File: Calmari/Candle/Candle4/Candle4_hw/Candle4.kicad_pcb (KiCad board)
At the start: 2 copper layers, 124 x 15 mm, 56 parts, among them Q1 LED_RGB, SW1 BUTTON, SW2 BUTTON, SW3 BUTTON

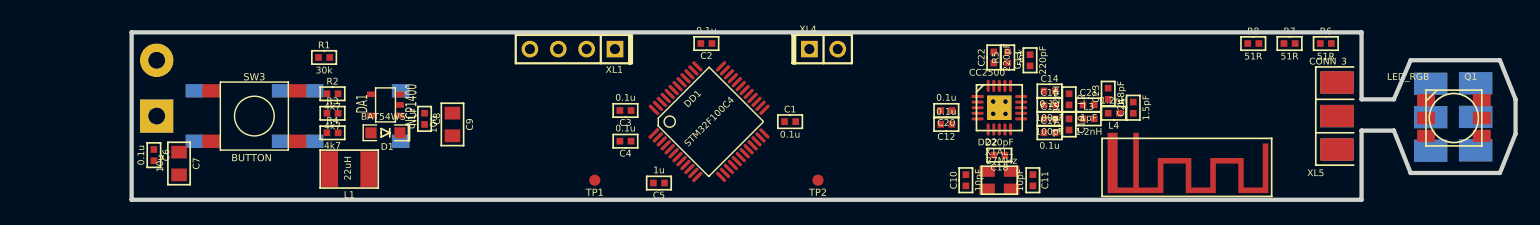
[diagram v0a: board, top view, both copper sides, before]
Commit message: gerber added
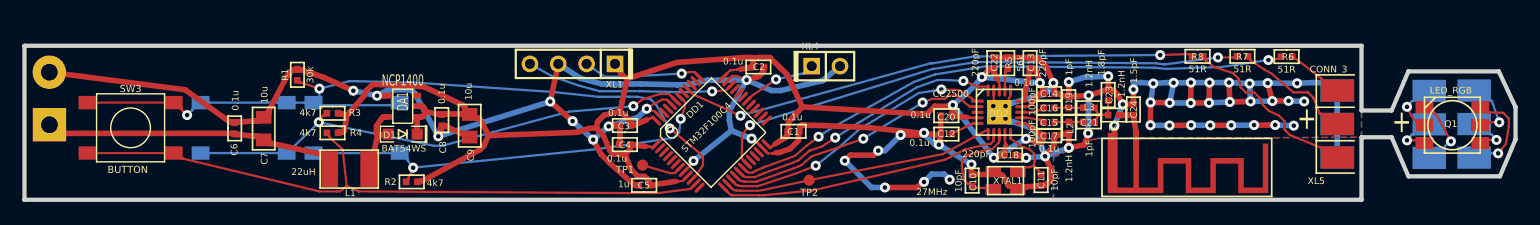
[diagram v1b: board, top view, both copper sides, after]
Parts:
- moved SW3 11.1 mm to (45.9, 70.6)
- moved R2 10.6 mm to (71.1, 75.4)
- moved XL3 9.68 mm to (38.6, 65.6)
- moved XL2 9.64 mm to (38.6, 70.3)
- moved C7 8.21 mm to (57.8, 70.6), turned to 90 degrees
- moved C6 7.62 mm to (55.2, 70.6), turned to 90 degrees
- moved R8 5.12 mm to (141.5, 64.1)
- moved C2 5.11 mm to (102.2, 65.1), turned to 0 degrees
- moved TP1 4.49 mm to (91.8, 73.9)
- moved R7 4.37 mm to (145.5, 64.1)
- moved R6 3.71 mm to (149.5, 64.2)
- moved R1 2.85 mm to (60.9, 65.8), turned to 90 degrees
- moved L2 2.53 mm to (130.0, 70.5), turned to 90 degrees
- moved C19 1.99 mm to (130.0, 68.3), turned to 90 degrees
- moved C8 1.55 mm to (73.8, 69.9)
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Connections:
- ANT1 pad 1: GND -> N-0000035
- C24 pad 1: GND -> N-0000035
- L4 pad 1: GND -> N-0000035
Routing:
- net GND: track 0.00 -> 308.6 mm, vias 0 -> 56
- net +3.3V: track 0.00 -> 160.3 mm, vias 0 -> 5
- net /WKUP: track 0.00 -> 71.9 mm, vias 0 -> 3
- net /BTN_TX: track 0.00 -> 60.9 mm
- net /LED_R: track 0.00 -> 50.9 mm, vias 0 -> 2
- net /LED_G: track 0.00 -> 48.4 mm, vias 0 -> 2
- net /LED_B: track 0.00 -> 46.6 mm, vias 0 -> 2
- net /BTN_DOWN: track 0.00 -> 46.1 mm, vias 0 -> 2
- net /BTN_UP: track 0.00 -> 38.6 mm, vias 0 -> 2
- net /BATT: track 0.00 -> 26.6 mm
- net /CC_CS: track 0.00 -> 25.8 mm
- net /CC_MOSI: track 0.00 -> 25.2 mm, vias 0 -> 2
- net /CC_SCK: track 0.00 -> 25.1 mm, vias 0 -> 2
- net /CC_GDO0: track 0.00 -> 24.9 mm
- net /CC_MISO: track 0.00 -> 24.2 mm, vias 0 -> 2
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- added copper zone on B.Cu, net GND
- added copper zone on F.Cu, net GND
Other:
- board size 124 x 15 mm -> 133.6 x 13.8 mm
- board text added: "+"
